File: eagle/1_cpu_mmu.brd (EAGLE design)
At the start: 160 x 100 mm, 47 parts, among them IC1 MT5C6408, IC10 74LS157N, IC11 74LS157N, IC12 74LS00N, IC13 74LS157N, IC14 74LS157N, IC17 74LS32N, IC19 74LS32N, IC2 MT5C6408, IC20 74LS02N, IC21 74LS374N, IC3 74LS27N, IC4 74LS20N, IC5 74LS08N, IC6 74LS245N, IC7 74LS245N, IC8 74LS32N, IC9 74LS157N

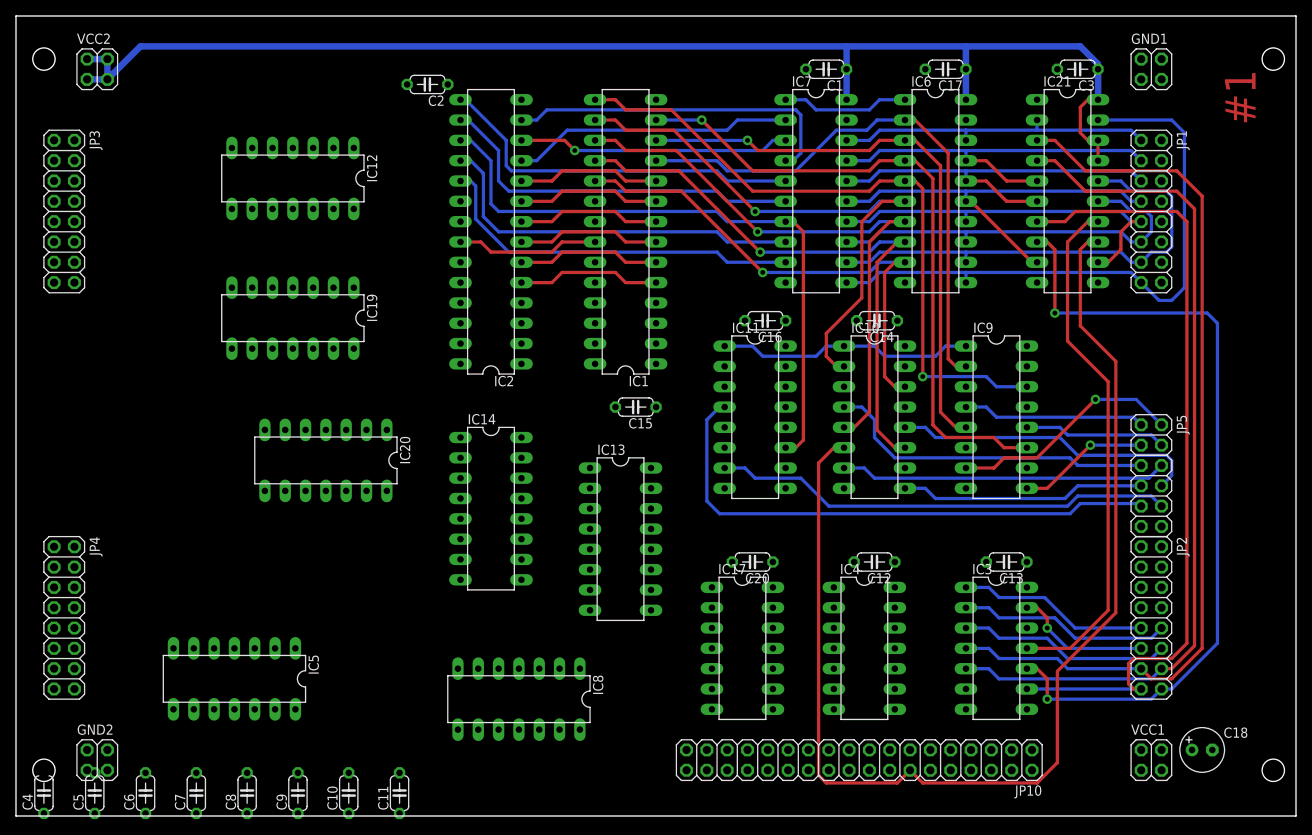
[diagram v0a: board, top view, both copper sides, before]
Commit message: MMU board updates 2016-03-16
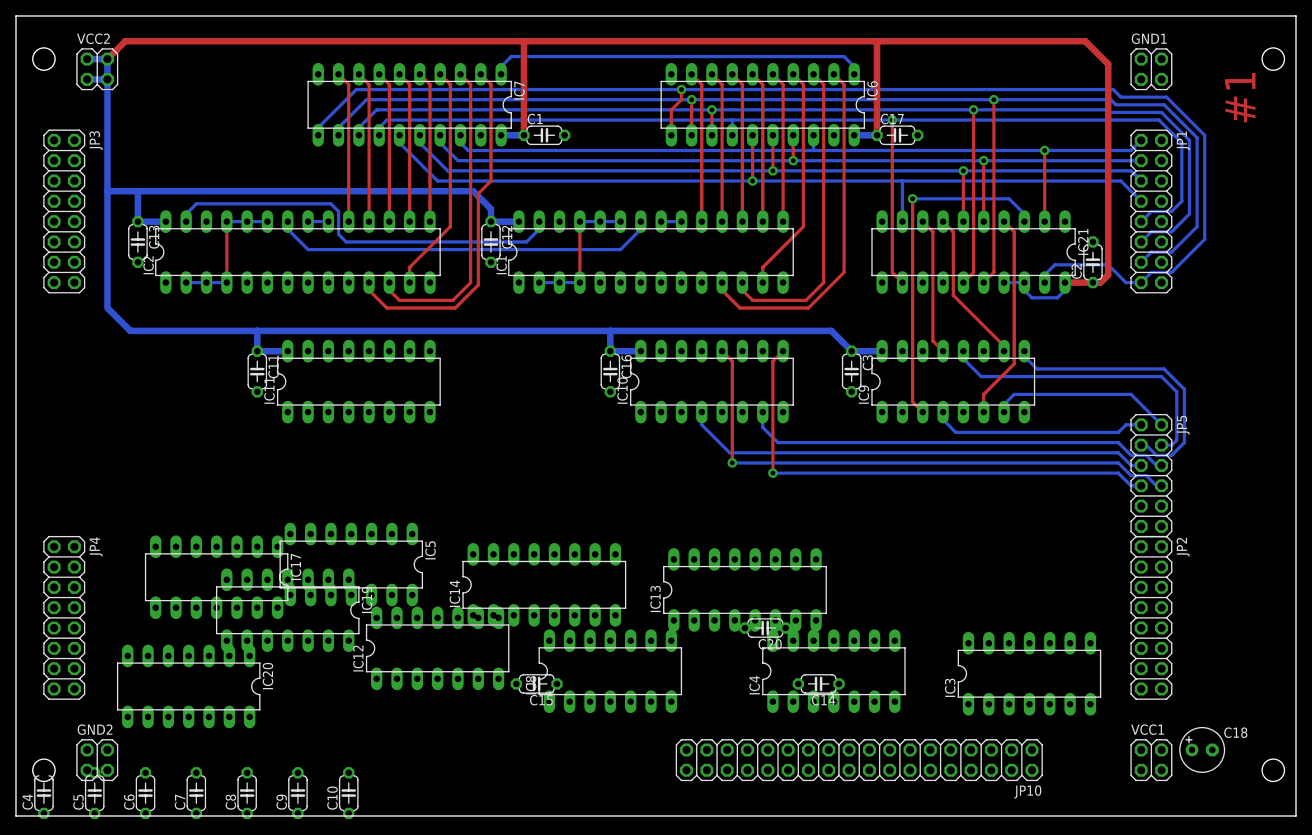
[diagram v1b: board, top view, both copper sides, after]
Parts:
- moved C13 115.7 mm to (15.2, 71.8), turned to 270 degrees
- moved C2 86.1 mm to (134.6, 69.2), turned to 90 degrees
- moved IC17 66.3 mm to (25.1, 29.8), turned to 180 degrees
- moved C12 62.4 mm to (59.4, 71.8), turned to 270 degrees
- moved IC12 61.5 mm to (52.7, 21.0), turned to 0 degrees
- moved C11 55.6 mm to (30.2, 55.6), turned to 270 degrees
- moved IC7 51.9 mm to (49.2, 88.9), turned to 180 degrees
- moved IC11 49.7 mm to (42.9, 54.3), turned to 0 degrees
- moved C3 47.2 mm to (104.5, 55.6), turned to 270 degrees
- moved C14 46.0 mm to (100.3, 16.5)
- moved C15 36.8 mm to (65.1, 16.5)
- moved IC19 36.5 mm to (34.0, 25.7)
- moved C1 36.2 mm to (66.0, 85.1), turned to 0 degrees
- moved IC20 33.1 mm to (21.6, 16.2)
- moved IC2 24.3 mm to (35.2, 70.5), turned to 0 degrees
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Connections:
- net ABUS0: now also IC12.1
- net ABUS12: now also IC9.3
- net ABUS13: now also IC9.6
- net ABUS14: now also IC9.10
- net ABUS15: now also IC9.13
- net GND: no longer IC9.10, IC9.13, IC9.3, IC9.6
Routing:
- net +5V: track 162.8 -> 407.8 mm
- net MEMSEG: track 147.2 -> 0.00 mm
- net DBUS6: track 60.1 -> 159.5 mm, vias 0 -> 2
- net DBUS5: track 50.3 -> 149.3 mm, vias 0 -> 2
- net DBUS4: track 48.0 -> 139.0 mm, vias 0 -> 1
- net ABUS15: track 101.2 -> 17.2 mm, vias 2 -> 0
- net DBUS7: track 76.9 -> 160.0 mm, vias 0 -> 1
- net ABUS13: track 107.6 -> 25.9 mm
- net ABUS14: track 99.5 -> 19.3 mm
- net ABUS12: track 112.7 -> 42.9 mm, vias 0 -> 1
- net PABUS20: track 68.6 -> 0.00 mm
- net /FS: track 65.1 -> 0.00 mm
- net N$8: track 83.7 -> 18.9 mm, vias 1 -> 0
- net /FIO: track 79.4 -> 18.9 mm
- net PABUS21: track 57.6 -> 0.00 mm
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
